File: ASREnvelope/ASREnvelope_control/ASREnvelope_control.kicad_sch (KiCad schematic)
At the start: 19 parts, among them J1 GATE, J3 OUT, J4 INV OUT, J5 Conn_01x06_Male, J6 Conn_01x04_Male, SW1 SW_SPDT

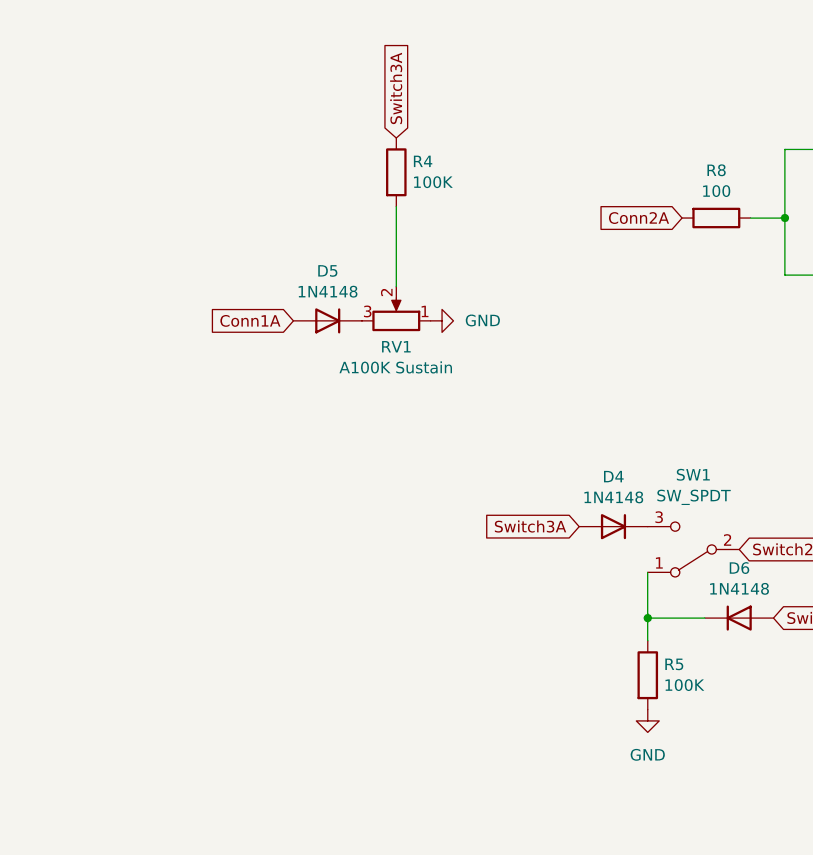
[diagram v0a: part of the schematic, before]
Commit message: fix errors
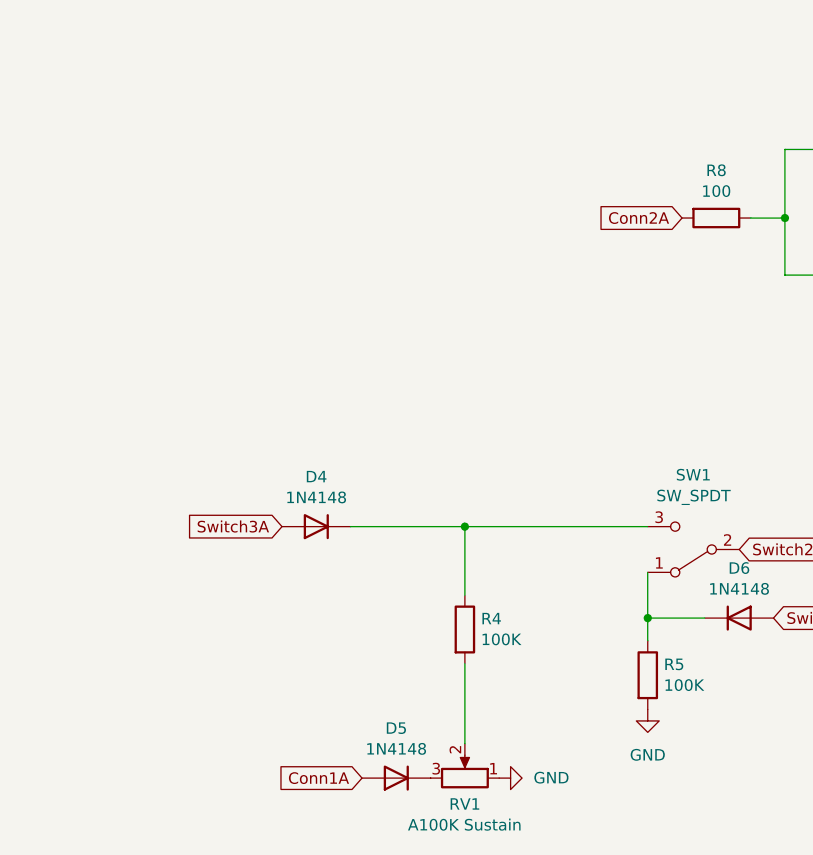
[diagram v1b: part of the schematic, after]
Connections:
- net Switch3A: no longer R4.1
- net at D4.1 (K), SW1.3 (C): now also R4.1
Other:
- moved on the sheet: D4, D5, R4, RV1
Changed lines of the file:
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@@
   (junction (at 170.18 39.37) (diameter 0) (color 0 0 0 0)
+  )
+  (junction (at 134.62 73.66) (diameter 0) (color 0 0 0 0)
   )
   (junction (at 195.58 45.72) (diameter 0) (color 0 0 0 0)
@@
   (no_connect (at 58.42 97.79))
   (no_connect (at 58.42 80.01))
+  (wire (pts (xy 121.92 73.66) (xy 134.62 73.66))
+    (stroke (width 0) (type default) (color 0 0 0 0))
+  )
   (wire (pts (xy 154.94 83.82) (xy 154.94 78.74))
     (stroke (width 0) (type default) (color 0 0 0 0))
   )
-  (wire (pts (xy 127 46.99) (xy 127 38.1))
+  (wire (pts (xy 134.62 97.79) (xy 134.62 88.9))
     (stroke (width 0) (type default) (color 0 0 0 0))
   )
@@
     (stroke (width 0) (type default) (color 0 0 0 0))
   )
+  (wire (pts (xy 134.62 73.66) (xy 154.94 73.66))
+    (stroke (width 0) (type default) (color 0 0 0 0))
+  )
   (wire (pts (xy 166.37 39.37) (xy 170.18 39.37))
+    (stroke (width 0) (type default) (color 0 0 0 0))
+  )
+  (wire (pts (xy 134.62 73.66) (xy 134.62 81.28))
     (stroke (width 0) (type default) (color 0 0 0 0))
   )
@@
     (effects (font (size 1.27 1.27)) (justify left))
     (property "Intersheet References" "${INTERSHEET_REFS}" (id 0) (at 76.2 -15.24 0)
-      (effects (font (size 1.27 1.27)) hide)
-    )
-  )
-  (global_label "Switch3A" (shape input) (at 127 30.48 90) (fields_autoplaced)
-    (effects (font (size 1.27 1.27)) (justify left))
-    (property "Intersheet References" "${INTERSHEET_REFS}" (id 0) (at 40.64 -48.26 0)
       (effects (font (size 1.27 1.27)) hide)
     )
@@
     )
   )
-  (global_label "Conn1A" (shape input) (at 115.57 50.8 180) (fields_autoplaced)
+  (global_label "Conn1A" (shape input) (at 123.19 101.6 180) (fields_autoplaced)
     (effects (font (size 1.27 1.27)) (justify right))
-    (property "Intersheet References" "${INTERSHEET_REFS}" (id 0) (at 40.64 -48.26 0)
+    (property "Intersheet References" "${INTERSHEET_REFS}" (id 0) (at 48.26 2.54 0)
       (effects (font (size 1.27 1.27)) hide)
     )
@@
     )
   )
-  (global_label "Switch3A" (shape input) (at 147.32 73.66 180) (fields_autoplaced)
+  (global_label "Switch3A" (shape input) (at 114.3 73.66 180) (fields_autoplaced)
     (effects (font (size 1.27 1.27)) (justify right))
-    (property "Intersheet References" "${INTERSHEET_REFS}" (id 0) (at 38.1 -31.75 0)
+    (property "Intersheet References" "${INTERSHEET_REFS}" (id 0) (at 5.08 -31.75 0)
       (effects (font (size 1.27 1.27)) hide)
     )
@@
     (pin "TN")
   )
-  (symbol (lib_id "Device:D") (at 119.38 50.8 180) (unit 1)
-    (in_bom yes) (on_board yes)
-    (property "Reference" "D5" (id 0) (at 119.38 45.2882 0))
-    (property "Value" "1N4148" (id 1) (at 119.38 47.5996 0))
-    (property "Footprint" "Diode_THT:D_DO-35_SOD27_P7.62mm_Horizontal" (id 2) (at 119.38 50.8 0)
-      (effects (font (size 1.27 1.27)) hide)
-    )
-    (property "Datasheet" "~" (id 3) (at 119.38 50.8 0)
-      (effects (font (size 1.27 1.27)) hide)
-    )
-    (pin "1")
-    (pin "2")
-  )
-  (symbol (lib_id "Device:D") (at 151.13 73.66 180) (unit 1)
-    (in_bom yes) (on_board yes)
-    (property "Reference" "D4" (id 0) (at 151.13 68.1482 0))
-    (property "Value" "1N4148" (id 1) (at 151.13 70.4596 0))
-    (property "Footprint" "Diode_THT:D_DO-35_SOD27_P7.62mm_Horizontal" (id 2) (at 151.13 73.66 0)
-      (effects (font (size 1.27 1.27)) hide)
-    )
-    (property "Datasheet" "~" (id 3) (at 151.13 73.66 0)
-      (effects (font (size 1.27 1.27)) hide)
-    )
-    (pin "1")
-    (pin "2")
-  )
-  (symbol (lib_id "ASREnvelope-rescue:R_POT-Device") (at 127 50.8 270) (mirror x) (unit 1)
-    (in_bom yes) (on_board yes)
-    (property "Reference" "RV1" (id 0) (at 127 53.721 90))
-    (property "Value" "A100K Sustain" (id 1) (at 127 56.0324 90))
-    (property "Footprint" "Eurocad:Alpha9mmPot" (id 2) (at 127 50.8 0)
-      (effects (font (size 1.27 1.27)) hide)
-    )
-    (property "Datasheet" "~" (id 3) (at 127 50.8 0)
+  (symbol (lib_id "Device:D") (at 127 101.6 180) (unit 1)
+    (in_bom yes) (on_board yes)
+    (property "Reference" "D5" (id 0) (at 127 96.0882 0))
+    (property "Value" "1N4148" (id 1) (at 127 98.3996 0))
+    (property "Footprint" "Diode_THT:D_DO-35_SOD27_P7.62mm_Horizontal" (id 2) (at 127 101.6 0)
+      (effects (font (size 1.27 1.27)) hide)
+    )
+    (property "Datasheet" "~" (id 3) (at 127 101.6 0)
+      (effects (font (size 1.27 1.27)) hide)
+    )
+    (pin "1")
+    (pin "2")
+  )
+  (symbol (lib_id "Device:D") (at 118.11 73.66 180) (unit 1)
+    (in_bom yes) (on_board yes)
+    (property "Reference" "D4" (id 0) (at 118.11 68.1482 0))
+    (property "Value" "1N4148" (id 1) (at 118.11 70.4596 0))
+    (property "Footprint" "Diode_THT:D_DO-35_SOD27_P7.62mm_Horizontal" (id 2) (at 118.11 73.66 0)
+      (effects (font (size 1.27 1.27)) hide)
+    )
+    (property "Datasheet" "~" (id 3) (at 118.11 73.66 0)
+      (effects (font (size 1.27 1.27)) hide)
+    )
+    (pin "1")
+    (pin "2")
+  )
+  (symbol (lib_id "ASREnvelope-rescue:R_POT-Device") (at 134.62 101.6 270) (mirror x) (unit 1)
+    (in_bom yes) (on_board yes)
+    (property "Reference" "RV1" (id 0) (at 134.62 104.521 90))
+    (property "Value" "A100K Sustain" (id 1) (at 134.62 106.8324 90))
+    (property "Footprint" "Eurocad:Alpha9mmPot" (id 2) (at 134.62 101.6 0)
+      (effects (font (size 1.27 1.27)) hide)
+    )
+    (property "Datasheet" "~" (id 3) (at 134.62 101.6 0)
       (effects (font (size 1.27 1.27)) hide)
     )
@@
     (pin "3")
   )
-  (symbol (lib_id "Device:R") (at 127 34.29 0) (unit 1)
-    (in_bom yes) (on_board yes)
-    (property "Reference" "R4" (id 0) (at 128.778 33.1216 0)
+  (symbol (lib_id "Device:R") (at 134.62 85.09 0) (unit 1)
+    (in_bom yes) (on_board yes)
+    (property "Reference" "R4" (id 0) (at 136.398 83.9216 0)
       (effects (font (size 1.27 1.27)) (justify left))
     )
-    (property "Value" "100K" (id 1) (at 128.778 35.433 0)
+    (property "Value" "100K" (id 1) (at 136.398 86.233 0)
       (effects (font (size 1.27 1.27)) (justify left))
     )
-    (property "Footprint" "Resistor_THT:R_Axial_DIN0207_L6.3mm_D2.5mm_P7.62mm_Horizontal" (id 2) (at 125.222 34.29 90)
-      (effects (font (size 1.27 1.27)) hide)
-    )
-    (property "Datasheet" "~" (id 3) (at 127 34.29 0)
+    (property "Footprint" "Resistor_THT:R_Axial_DIN0207_L6.3mm_D2.5mm_P7.62mm_Horizontal" (id 2) (at 132.842 85.09 90)
+      (effects (font (size 1.27 1.27)) hide)
+    )
+    (property "Datasheet" "~" (id 3) (at 134.62 85.09 0)
       (effects (font (size 1.27 1.27)) hide)
     )
@@
     (pin "1")
   )
-  (symbol (lib_id "power:GND") (at 130.81 50.8 90) (unit 1)
-    (in_bom yes) (on_board yes) (fields_autoplaced)
-    (property "Reference" "#PWR0102" (id 0) (at 137.16 50.8 0)
-      (effects (font (size 1.27 1.27)) hide)
-    )
-    (property "Value" "GND" (id 1) (at 134.62 50.7999 90)
-      (effects (font (size 1.27 1.27)) (justify right))
-    )
-    (property "Footprint" "" (id 2) (at 130.81 50.8 0)
-      (effects (font (size 1.27 1.27)) hide)
-    )
-    (property "Datasheet" "" (id 3) (at 130.81 50.8 0)
-      (effects (font (size 1.27 1.27)) hide)
-    )
+  (symbol (lib_id "power:GND") (at 138.43 101.6 90) (unit 1)
+    (in_bom yes) (on_board yes) (fields_autoplaced)
+    (property "Reference" "#PWR0102" (id 0) (at 144.78 101.6 0)
+      (effects (font (size 1.27 1.27)) hide)
+    )
+    (property "Value" "GND" (id 1) (at 142.24 101.5999 90)
+      (effects (font (size 1.27 1.27)) (justify right))
+    )
+    (property "Footprint" "" (id 2) (at 138.43 101.6 0)
+      (effects (font (size 1.27 1.27)) hide)
+    )
+    (property "Datasheet" "" (id 3) (at 138.43 101.6 0)
+      (effects (font (size 1.27 1.27)) hide)
+    )
